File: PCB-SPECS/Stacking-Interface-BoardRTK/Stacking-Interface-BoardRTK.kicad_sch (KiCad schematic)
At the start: 0 parts

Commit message: Update
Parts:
- added ESP_Left, ESP_Right: Conn_01x15_Socket, symbol Connector:Conn_01x15_Socket
- added RTK_Bottom_Left: Conn_01x10_Pin, symbol Connector:Conn_01x10_Pin
- added RTK_Bottom_Right, RTK_Top_Left: Conn_01x08_Pin, symbol Connector:Conn_01x08_Pin
- added RTK_Top_Right: Conn_01x06_Pin, symbol Connector:Conn_01x06_Pin

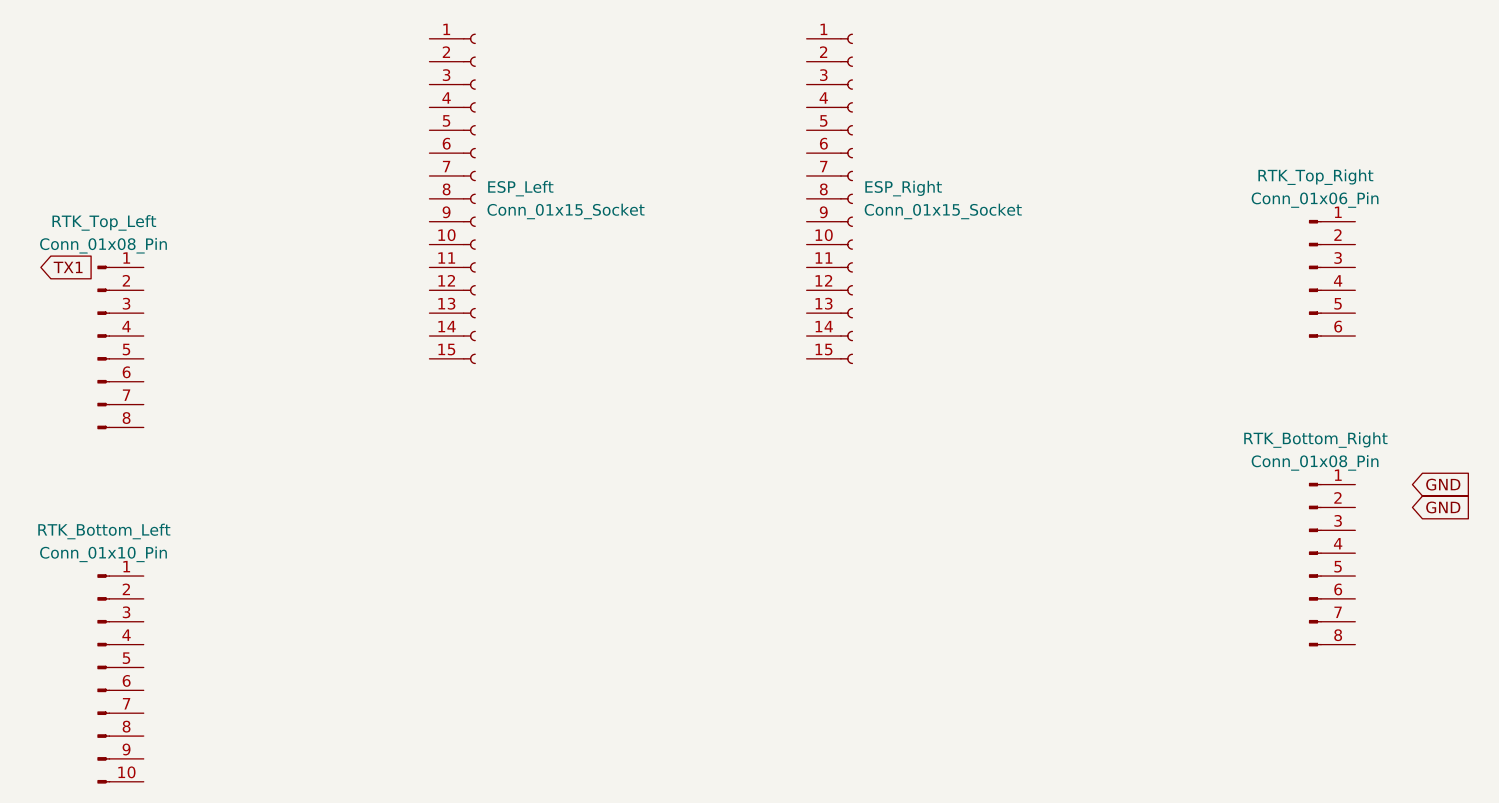
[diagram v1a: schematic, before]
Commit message: updates
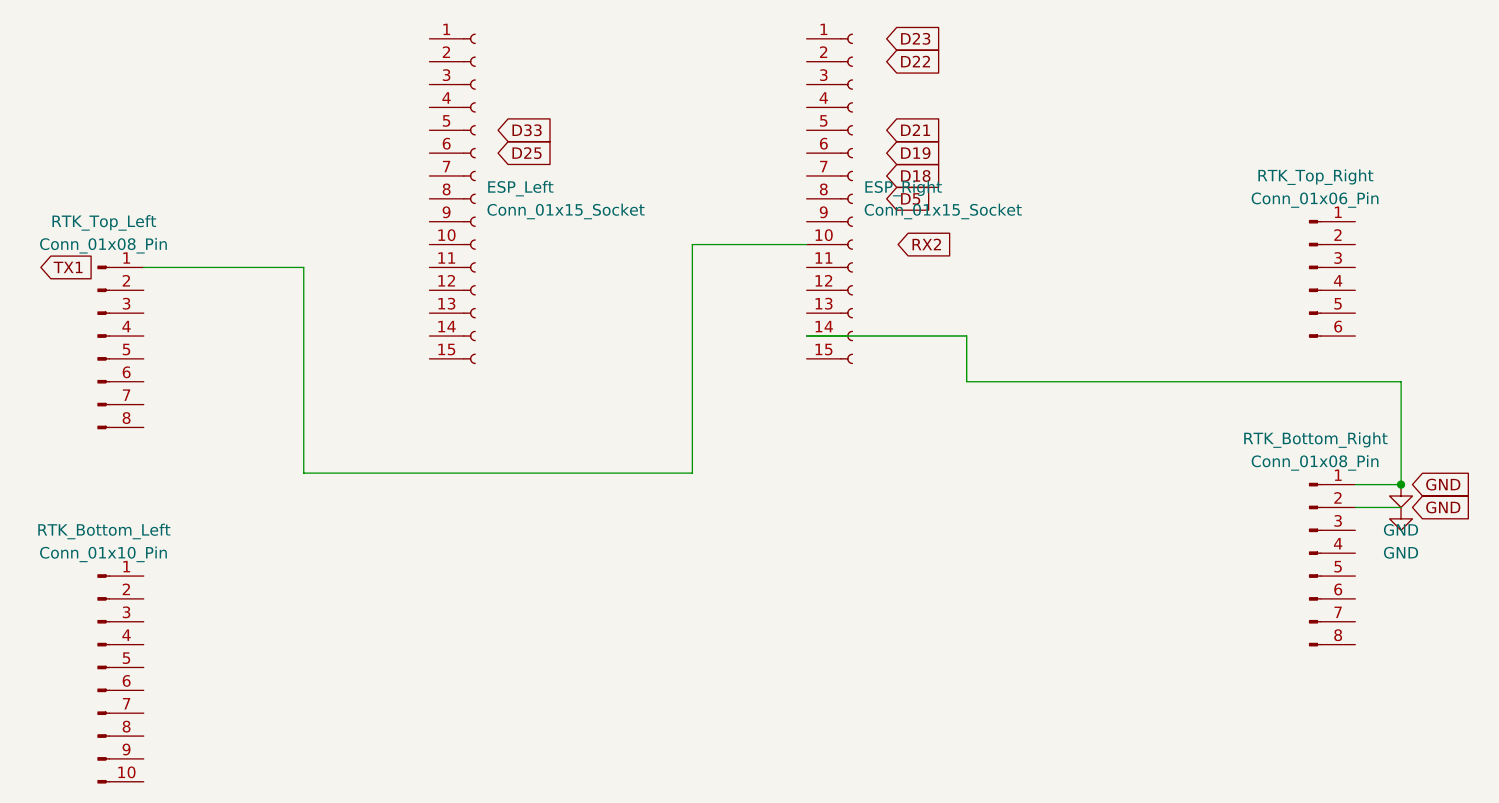
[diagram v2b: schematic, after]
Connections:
- net GND: now also ESP_Right.14 (Pin_14), RTK_Bottom_Right.1 (Pin_1), RTK_Bottom_Right.2 (Pin_2)
- net at ESP_Right.10 (Pin_10): now also RTK_Top_Left.1 (TX1)
